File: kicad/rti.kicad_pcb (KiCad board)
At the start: 2 copper layers, 100 x 80 mm, 58 parts, among them J1 Phoenix MKDS, J10 Header 2x3, J11 JST PH 4, J2 NRJ6HF, J3 NRJ6HF, J4 MEBP 8-8G, J5 MEBP 8-8G, J6 JST PH 3, J7 JST PH 3, J8 JST PH 3, J9 JST PH 3, M3 MountingHole_3.2mm_M3_DIN965, M3_2 MountingHole_3.2mm_M3_DIN965, M3_3 MountingHole_3.2mm_M3_DIN965, Q1 BD140, Q10 BD140, Q11 BD140, Q12 BD140, Q13 BD140, Q14 BD140, Q15 BD140, Q16 BD140, Q2 BD140, Q3 BD140, Q4 BD140, Q5 BD140, Q6 BD140, Q7 BD140, Q8 BD140, Q9 BD140, SW1 Switch, SW2 Switch, U1 ATMEGA328-PU, U2 TPIC6B595N, U3 TPIC6B595N, U4 PC827, U5 LM317T, U6 L7805CV, Y1 16MHz

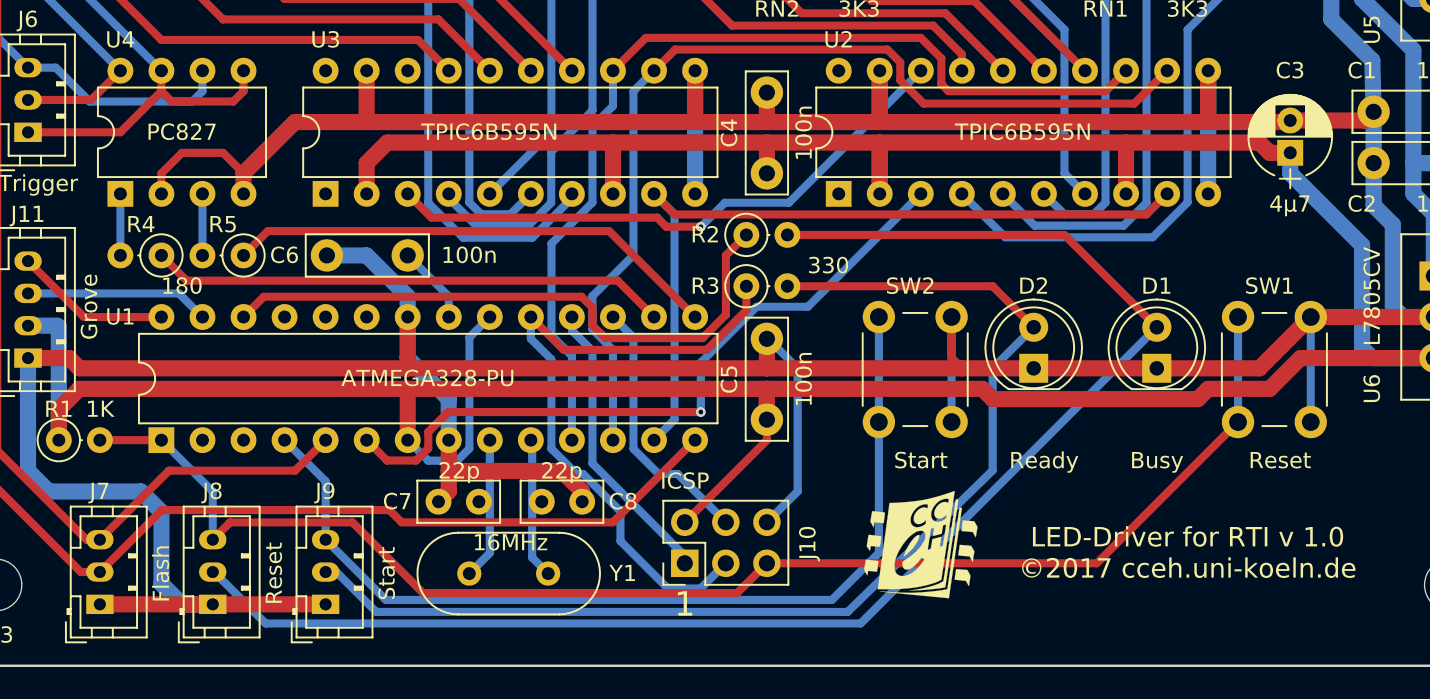
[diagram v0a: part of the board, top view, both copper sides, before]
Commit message: Update kicad format
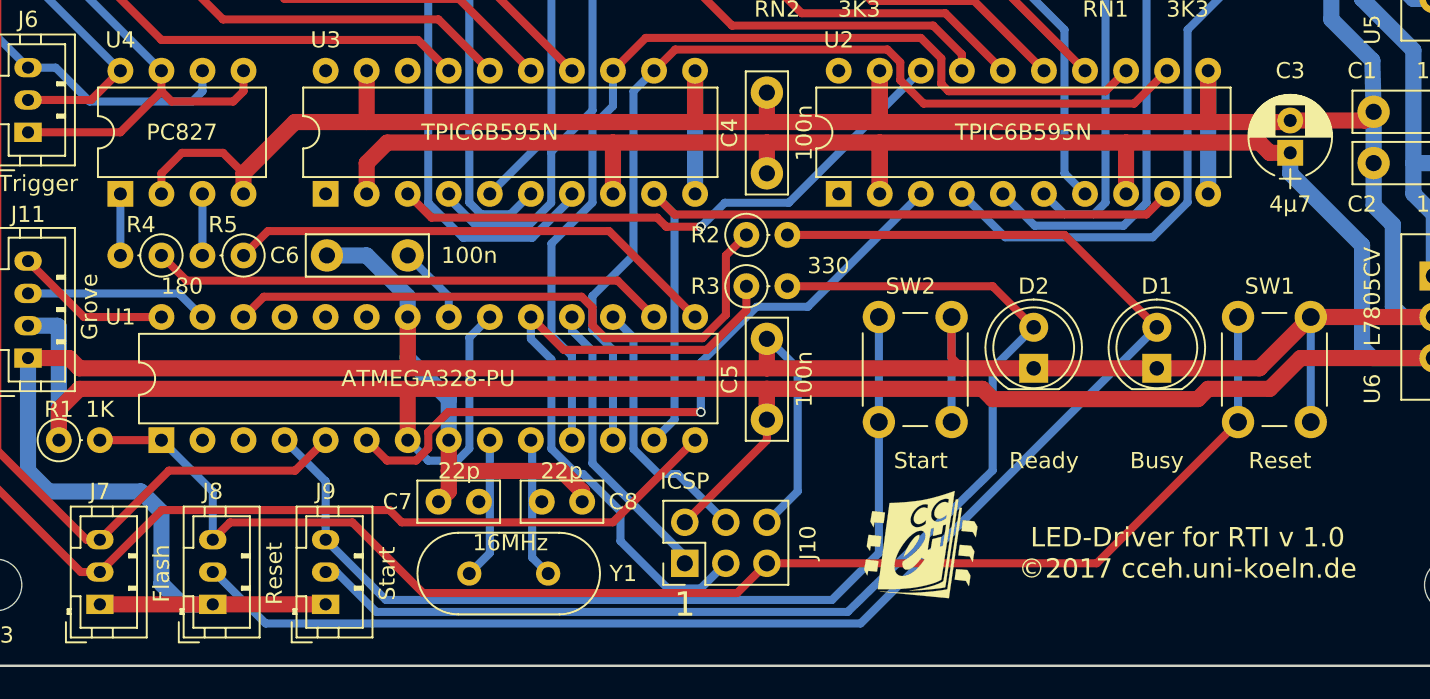
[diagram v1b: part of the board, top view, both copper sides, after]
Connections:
- net /~RESET renamed /~{RESET}
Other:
- net class +5V removed
- net class Default removed
- net class HC removed
- net class HC2HC removed
